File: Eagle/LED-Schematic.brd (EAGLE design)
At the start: 80 x 75.9 mm, 8 parts, among them Q1 INFINEON_IRLB8721PBFINFINEON_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, Q2 INFINEON_IRLB8721PBFINFINEON_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, Q3 INFINEON_IRLB8721PBFINFINEON_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, X1 DG3XX-03-3.5, X2 DG3XX-03-3.5, X3 DG3XX-03-3.5, X4 DG3XX-03-3.5

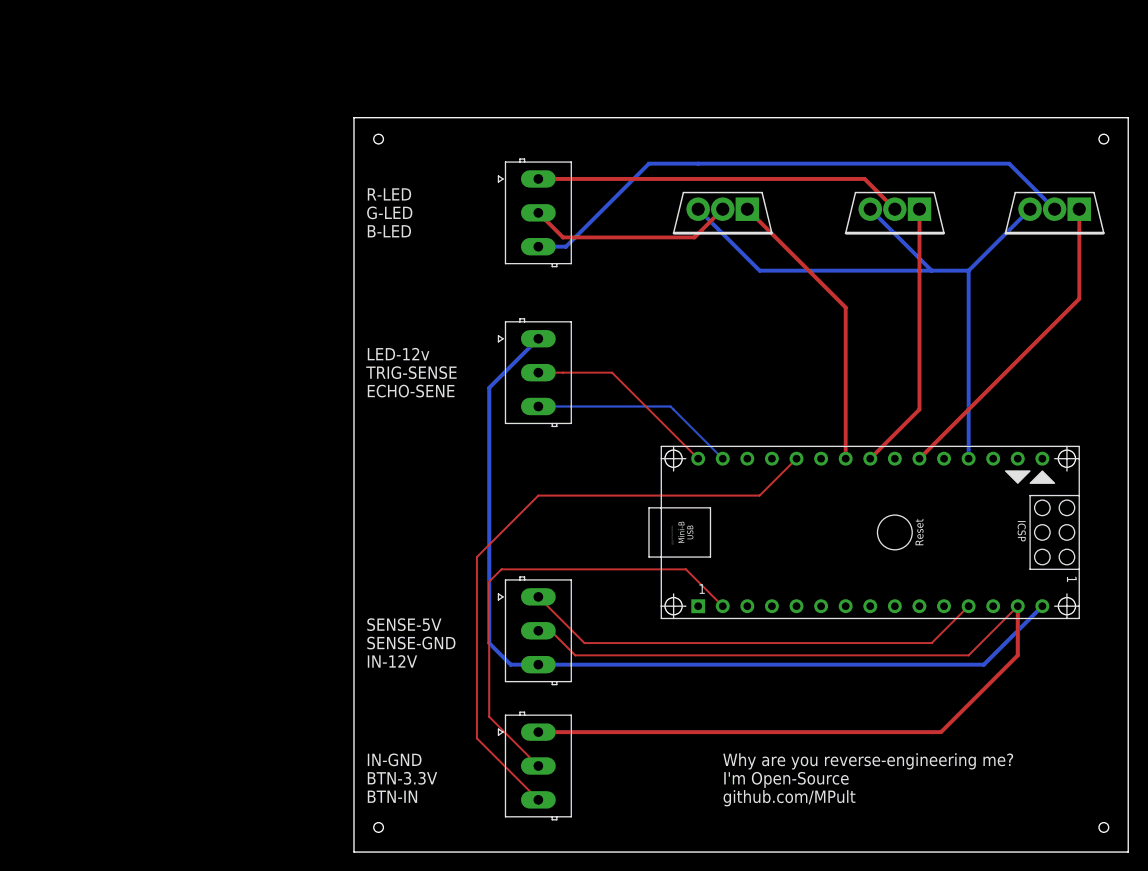
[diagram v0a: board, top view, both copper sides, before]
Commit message: Integrated
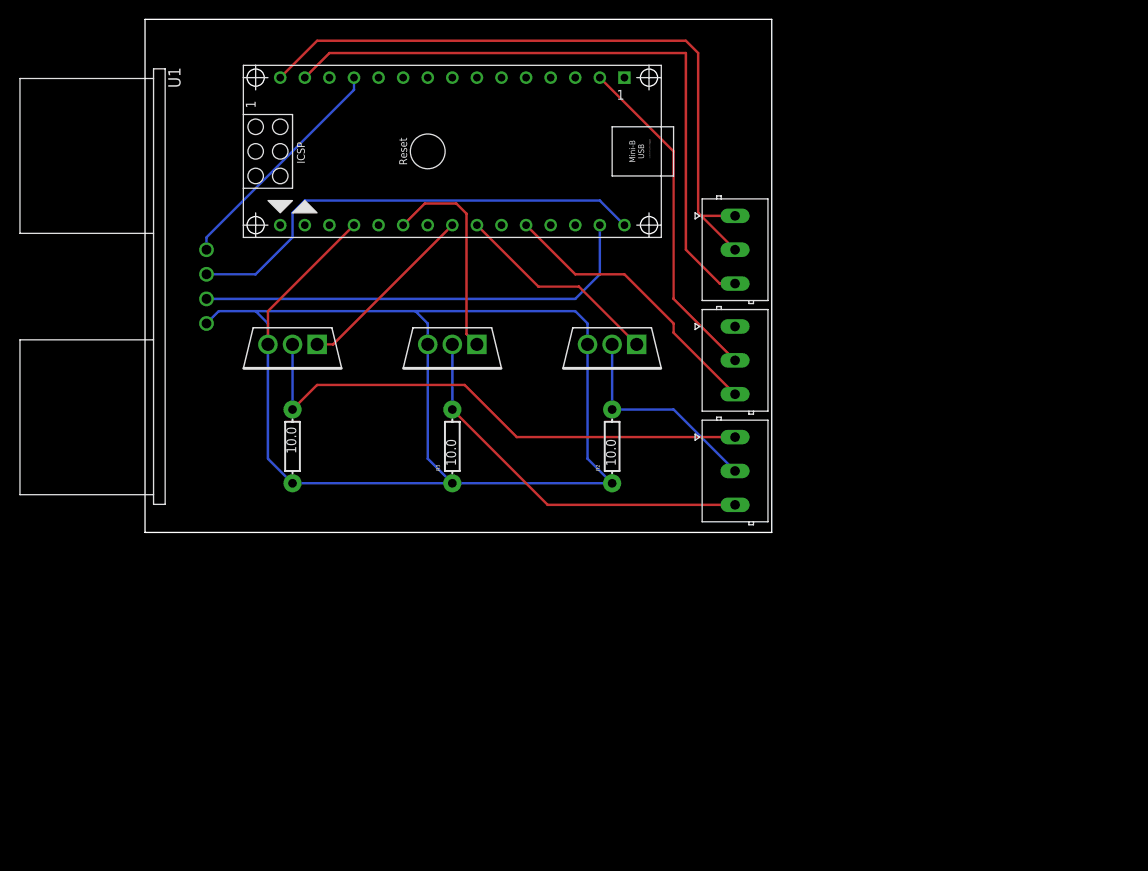
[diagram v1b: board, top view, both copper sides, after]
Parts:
- removed X3: DG3XX-03-3.5, degson:DG350-3.5-03P
- added R1, R2, R3: 10.0, SparkFun-Resistors:AXIAL-0.3
- added U1: HC-SR04, HC-SR04:XCVR_HC-SR04
- moved Q1 63.8 mm to (-17.8, 78.7)
- moved Q3 63.8 mm to (-1.27, 78.7)
- moved ARDUINO_NANO1 62.3 mm to (-3.81, 99.1), turned to 180 degrees
- moved X4 46.6 mm to (27.9, 77.5)
- moved X1 33.5 mm to (27.9, 66.0)
- moved X2 24.0 mm to (27.9, 88.9)
- moved Q2 18.1 mm to (15.2, 78.7)
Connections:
- net 12V: now also X2.2; no longer X3.3
- net 5V: now also U1.1; no longer X3.1
- net B-LED: now also R3.P$2
- net ECHO-SENSE: now also U1.3; no longer X2.3
- net G-LED: now also R2.P$2
- net GND: now also R1.P$1, R2.P$1, R3.P$1, U1.4, X2.3; no longer X3.2, X4.1
- net R-LED: now also R1.P$2
- net TRIG-SENSE: now also U1.2; no longer X2.2
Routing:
- net BTN-IN: track 64.9 -> 29.4 mm
- net GND: track 178.5 -> 213.4 mm
- net TRIG-SENSE: track 20.2 -> 48.9 mm
- net ECHO-SENSE: track 21.3 -> 46.8 mm
- net 5V: track 48.0 -> 24.1 mm
- net 12V: track 94.1 -> 70.7 mm
- net B-LED: track 58.8 -> 40.0 mm
- net R-LED: track 38.1 -> 55.7 mm
- net 3.3V: track 47.4 -> 35.0 mm
- net B-GATE: track 32.6 -> 21.9 mm
- net R-GATE: track 27.9 -> 19.1 mm
- net G-GATE: track 30.0 -> 21.6 mm
- net G-LED: track 21.3 -> 22.1 mm
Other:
- board size 80 x 75.9 mm -> 64.8 x 53 mm
- board text removed: "IN-GND BTN-3.3V BTN-IN"
- board text removed: "JLCJLCJLCJLC"
- board text removed: "LED-12v TRIG-SENSE ECHO-SENE"
- board text removed: "Made in Space By Aliens"
- board text removed: "R-LED G-LED B-LED"
- board text removed: "SENSE-5V SENSE-GND IN-12V"
- board text removed: "Why are you reverse-engineering me? I'm Open-Source github.com/MPult"
